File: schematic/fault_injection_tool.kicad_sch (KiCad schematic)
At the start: 7 parts, among them J1 Conn_01x02_Pin, J2 Conn_01x02_Pin, Q1 2N7000

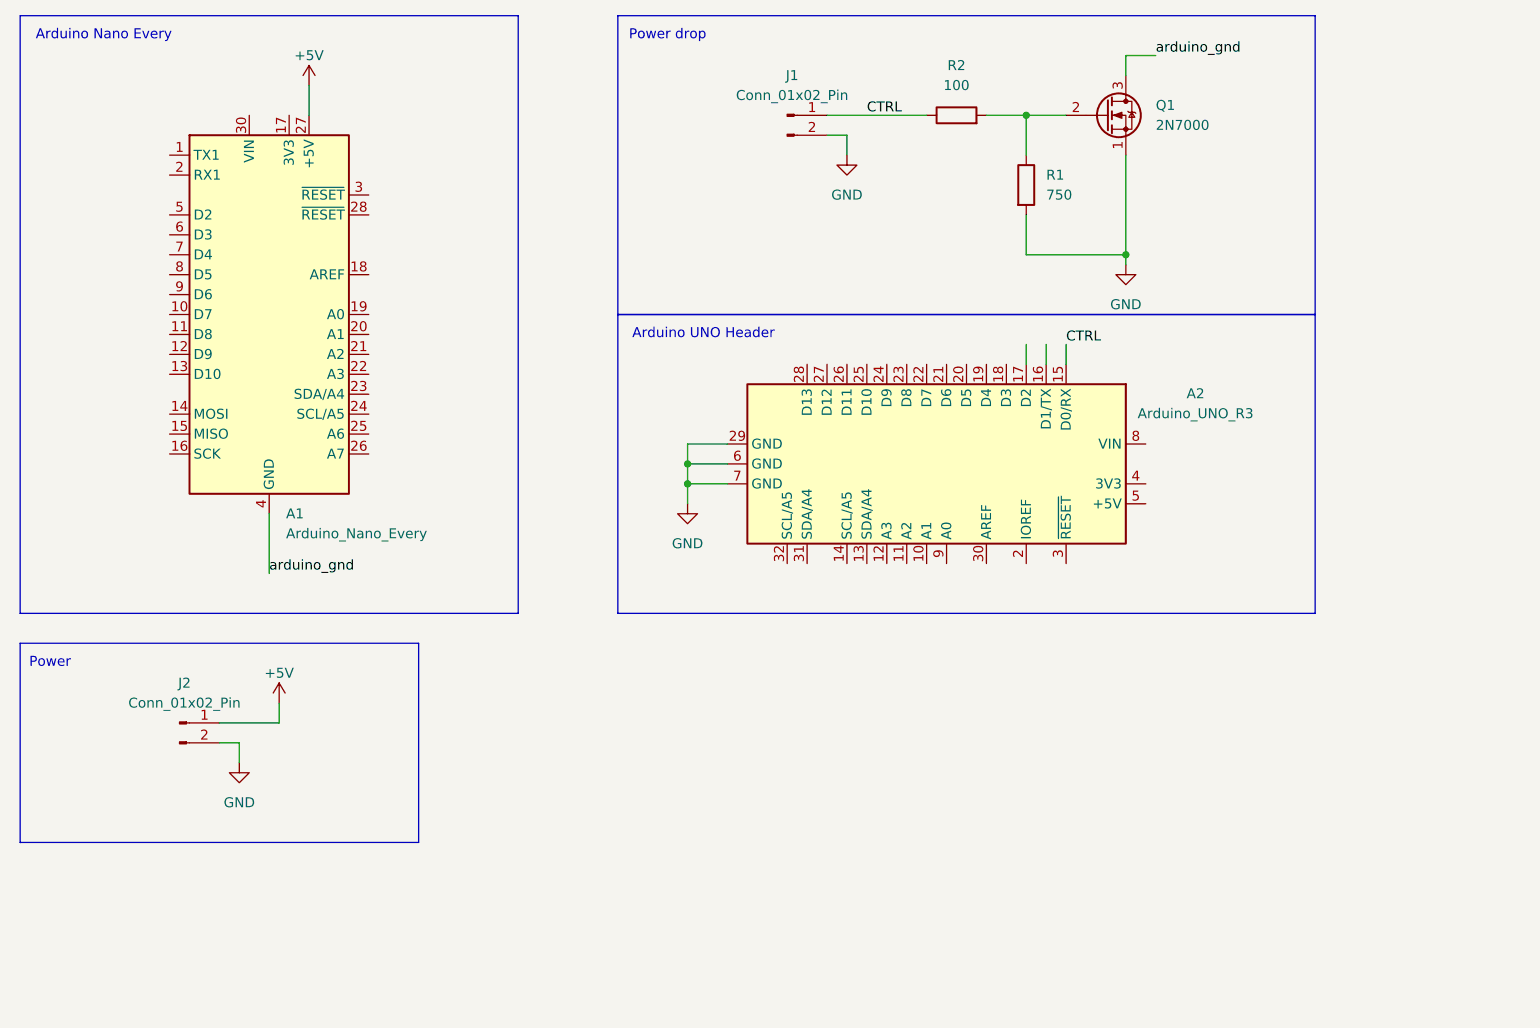
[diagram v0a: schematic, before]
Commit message: Updated schematic drawing and PCB design
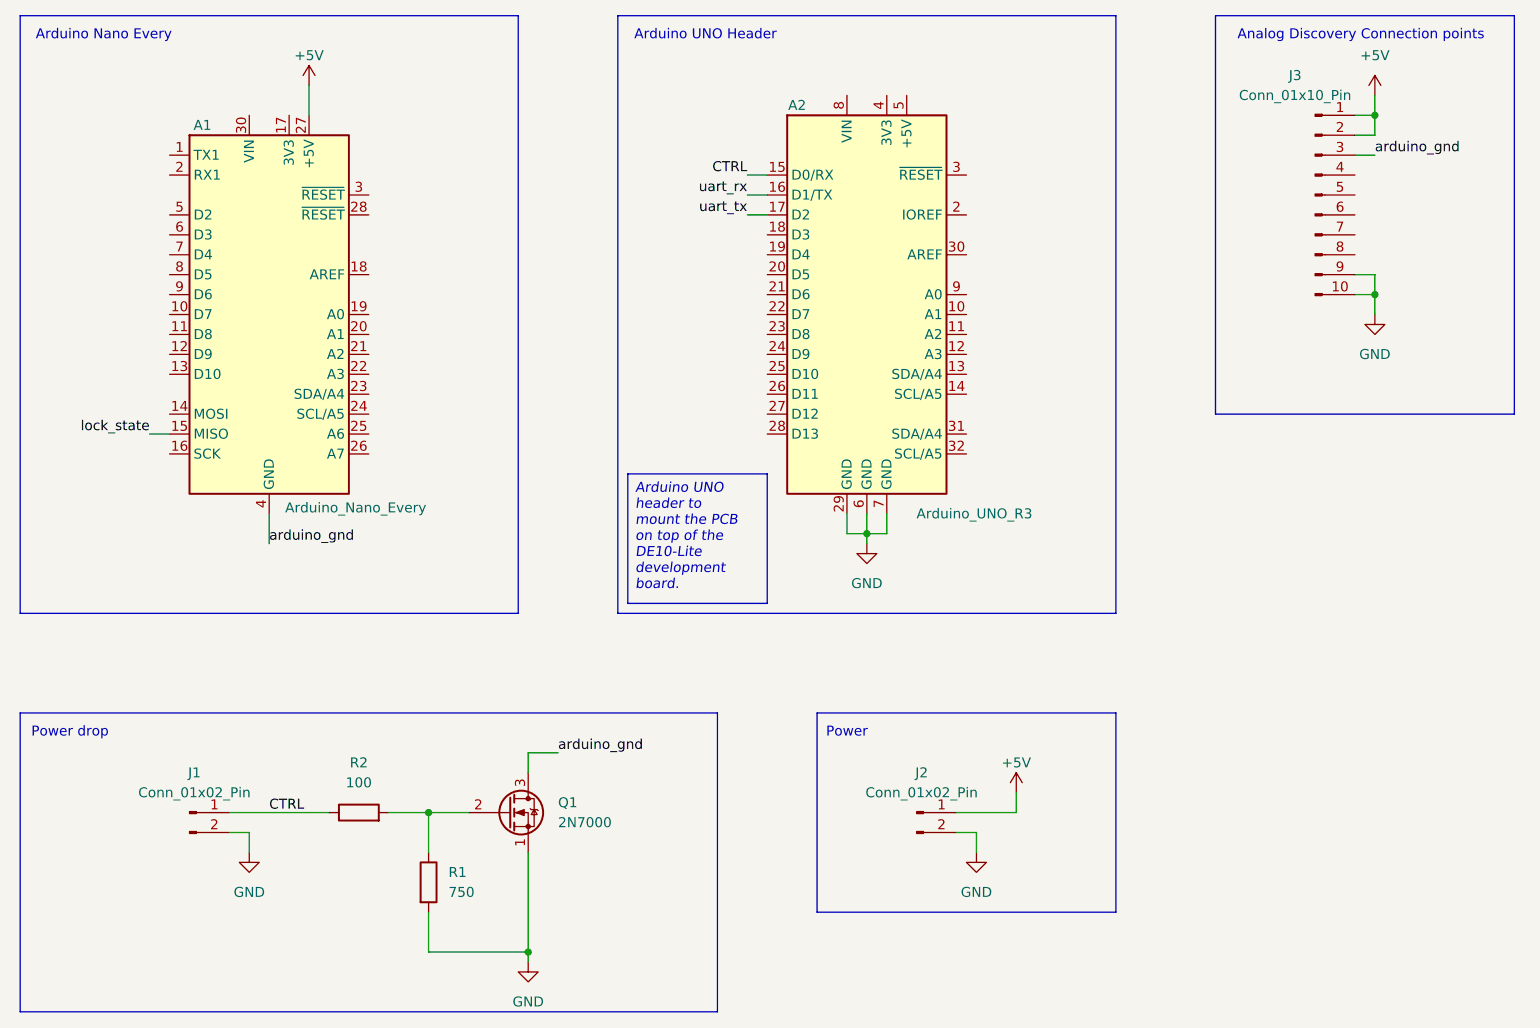
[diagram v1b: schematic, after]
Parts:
- added J3: Conn_01x10_Pin, symbol Connector:Conn_01x10_Pin
- R1, R2: footprint Resistor_SMD:R_0201_0603Metric_Pad0.64x0.40mm_HandSolder -> Resistor_SMD:R_0603_1608Metric_Pad0.98x0.95mm_HandSolder
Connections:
- net +5V: now also J3.1 (Pin_1), J3.2 (Pin_2)
- net GND: now also J3.10 (Pin_10), J3.9 (Pin_9)
- net arduino_gnd: now also J3.3 (Pin_3)
- net uart_rx: now reaches A2.16 (D1/TX)
- net uart_tx: now reaches A2.17 (D2)
- net lock_state: now reaches A1.15 (MISO)
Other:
- note added: "Analog Discovery Connection points"
- moved on the sheet: A2, J1, J2, Q1, R1, R2
